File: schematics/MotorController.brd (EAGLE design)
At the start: 124.4 x 96.2 mm, 37 parts, among them IC1 7805, Q1 BC307

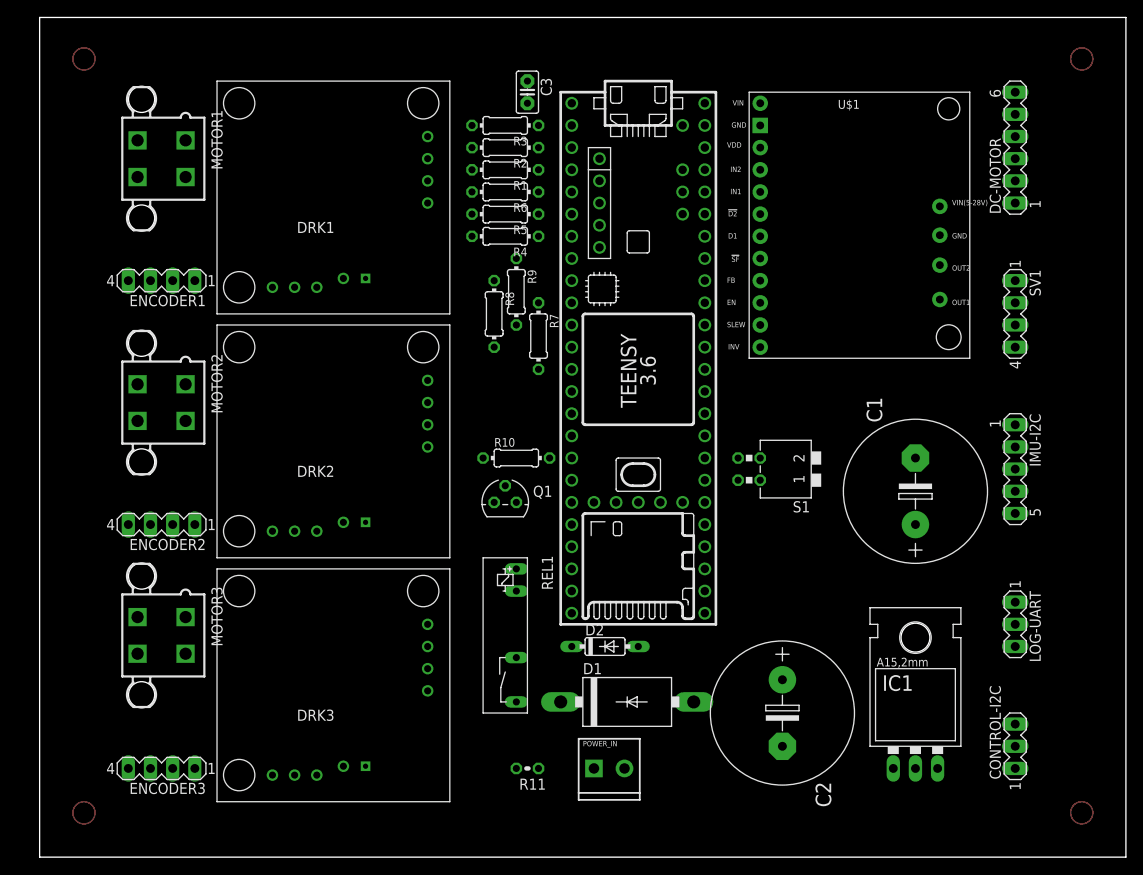
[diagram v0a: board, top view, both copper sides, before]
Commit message: no message
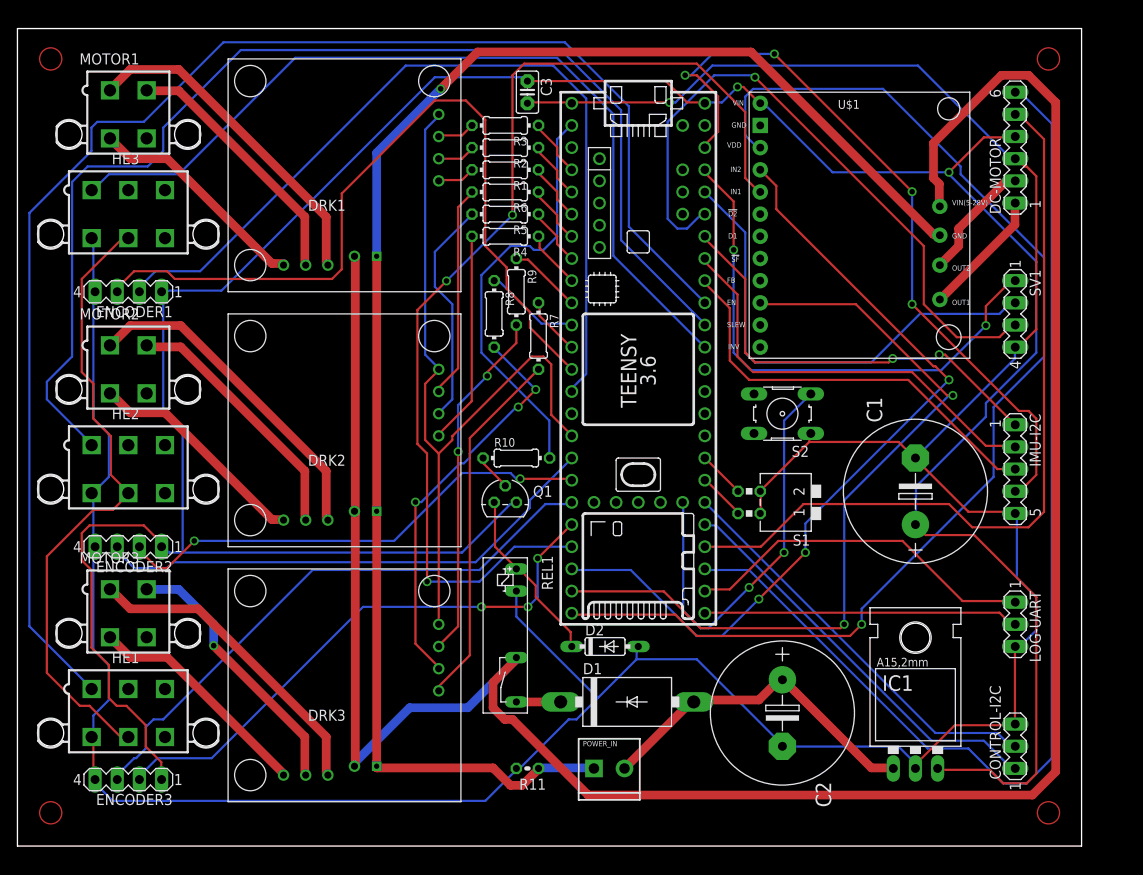
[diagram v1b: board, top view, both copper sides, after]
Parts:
- added HE1, HE2, HE3: 5566-6, con-molex:5566-6
- added S2: (no value), switch-omron:B3F-10XX
- moved MOTOR1 6.35 mm to (-62.2, 76.2), turned to 180 degrees
- moved MOTOR2 5.39 mm to (-62.2, 47.0), turned to 180 degrees
- moved ENCODER2 4.58 mm to (-62.2, 26.7)
- moved MOTOR3 4.58 mm to (-62.2, 19.1), turned to 180 degrees
- moved ENCODER3 4.02 mm to (-62.2, 0.00)
- moved ENCODER1 4.02 mm to (-62.2, 55.9)
- moved S1 3.81 mm to (8.89, 31.8)
- moved DRK1 2.84 mm to (-38.1, 69.8)
- moved DRK2 1.80 mm to (-38.1, 40.6)
- moved DRK3 1.27 mm to (-38.1, 11.4)
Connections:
- new net N$52: PRJ1.RESET, S2.3
- new net N$53: HE1.5, HE2.5, HE3.5
- new net N$54: HE1.1, PRJ1.17/A3
- new net N$55: HE2.1, PRJ1.16/A2
- new net N$56: HE3.1, PRJ1.15/A1
- net GND: now also HE1.4, HE2.4, HE3.4, S2.1, S2.2
- net N$42: now also PRJ1.0/RX
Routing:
- net GND: track 0.00 -> 374.7 mm, vias 0 -> 1
- net VCC: track 0.00 -> 334.1 mm, vias 0 -> 2
- net LIPO-VDD: track 0.00 -> 261.9 mm
- net LIPO-GND: track 0.00 -> 175.1 mm, vias 0 -> 1
- net N$54: track 0.00 -> 165.0 mm
- net N$55: track 0.00 -> 135.6 mm
- net N$41: track 0.00 -> 135.5 mm, vias 0 -> 1
- net WH_ENC_B: track 0.00 -> 129.5 mm
- net N$44: track 0.00 -> 120.7 mm, vias 0 -> 3
- net N$56: track 0.00 -> 99.7 mm
- net N$34: track 0.00 -> 98.1 mm
- net N$47: track 0.00 -> 93.7 mm, vias 0 -> 3
- net N$45: track 0.00 -> 91.3 mm, vias 0 -> 2
- net N$33: track 0.00 -> 90.9 mm
- net Y_ENC_A: track 0.00 -> 89.9 mm
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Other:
- board size 124.4 x 96.2 mm -> 121.9 x 93.7 mm
